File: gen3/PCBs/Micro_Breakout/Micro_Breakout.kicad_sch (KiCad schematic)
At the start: 49 parts, among them J1 BlueRobotics Depth Sensor, J10 Kill Switch, J11 StarOddi CTD Comms, J12 LED1, J13 LED2, J14 Leak Sensor, J15 Extra I2C #3, J16 Extra I2C #6, J17 Extra I2C #5, J18 Extra I2C #4, J19 GND Line, J2 Interconnect, J20 3.3V Line, J21 5V Line, J22 Extra SPI #1, J23 Extra SPI #2, J24 Extra SPI #3, J25 Secondary UART, J3 External Battery, J4 Conn_01x24, J5 External I2C, J6 Conn_01x24, J7 Extra I2C #1, J8 Extra I2C #2, J9 Lumen PWM, Q7 L78M05ABDT-TR, U1 SHT31-DIS-B, U15 AMS1117-3.3, U2 MCP9808_MSOP, U3 MS560702BA03-50, U6 Teensy4.1

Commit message: works
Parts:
- J1, J11, J15, J16, J17, J18, J25, J7, J8: footprint robosub_footprints:CONN_SD-43045-008_04_MOL -> robosub_footprints:CONN_SD-43045-005_04_MOL; symbol robosub_symbols:430450422 -> robosub_symbols:430450412; Supplier 1 https://www.digikey.com/en/products/detail/molex/0430450422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 -> https://www.digikey.com/en/products/detail/molex/0430450412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; Supplier 1 S/N WM2679-ND -> WM1790-ND
- J10, J12, J13, J9: footprint robosub_footprints:CONN_SD-43045-010_02_MOL -> robosub_footprints:CONN_SD-43045-005_02_MOL; symbol robosub_symbols:430450228 -> robosub_symbols:430450212; Supplier 1 https://www.digikey.com/en/products/detail/molex/0430450201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 -> https://www.digikey.com/en/products/detail/molex/0430450212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; Supplier 1 S/N WM9815-ND -> WM1789-ND
- J22, J23, J24: Supplier 1 (none) -> https://www.digikey.com/en/products/detail/molex/0430450612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; Supplier 1 S/N (none) -> WM1791-ND
- U6: footprint Imported_Footprints:Teensy41 -> robosub_footprints:Teensy41

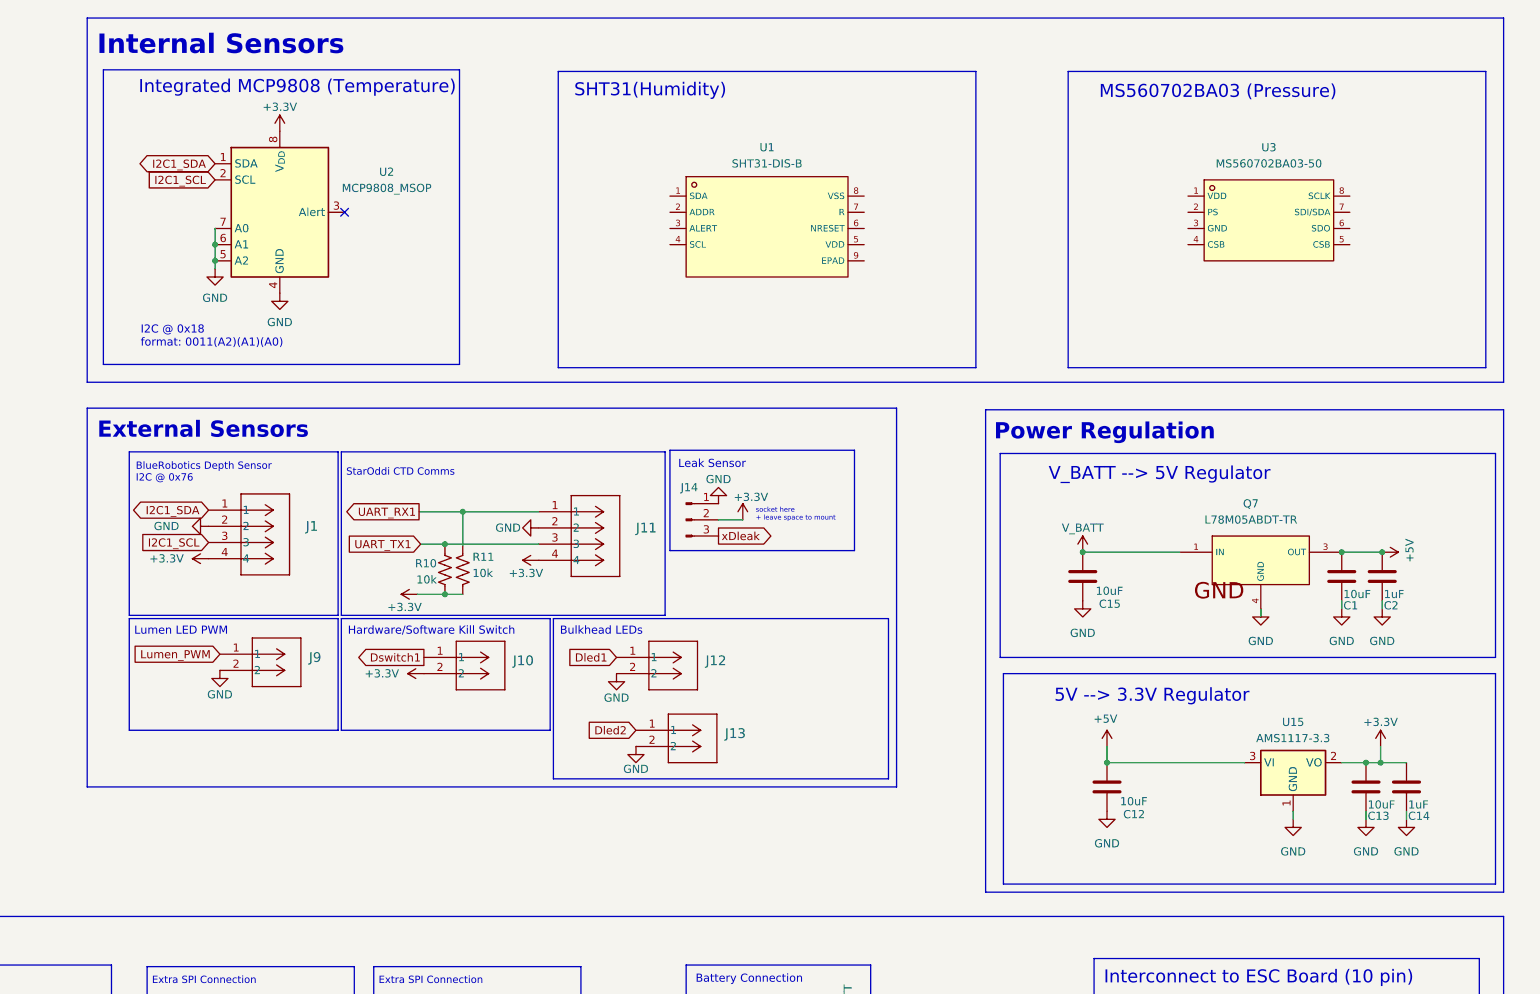
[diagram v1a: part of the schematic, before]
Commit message: jlc_to_robosub working, and all parts are updated.
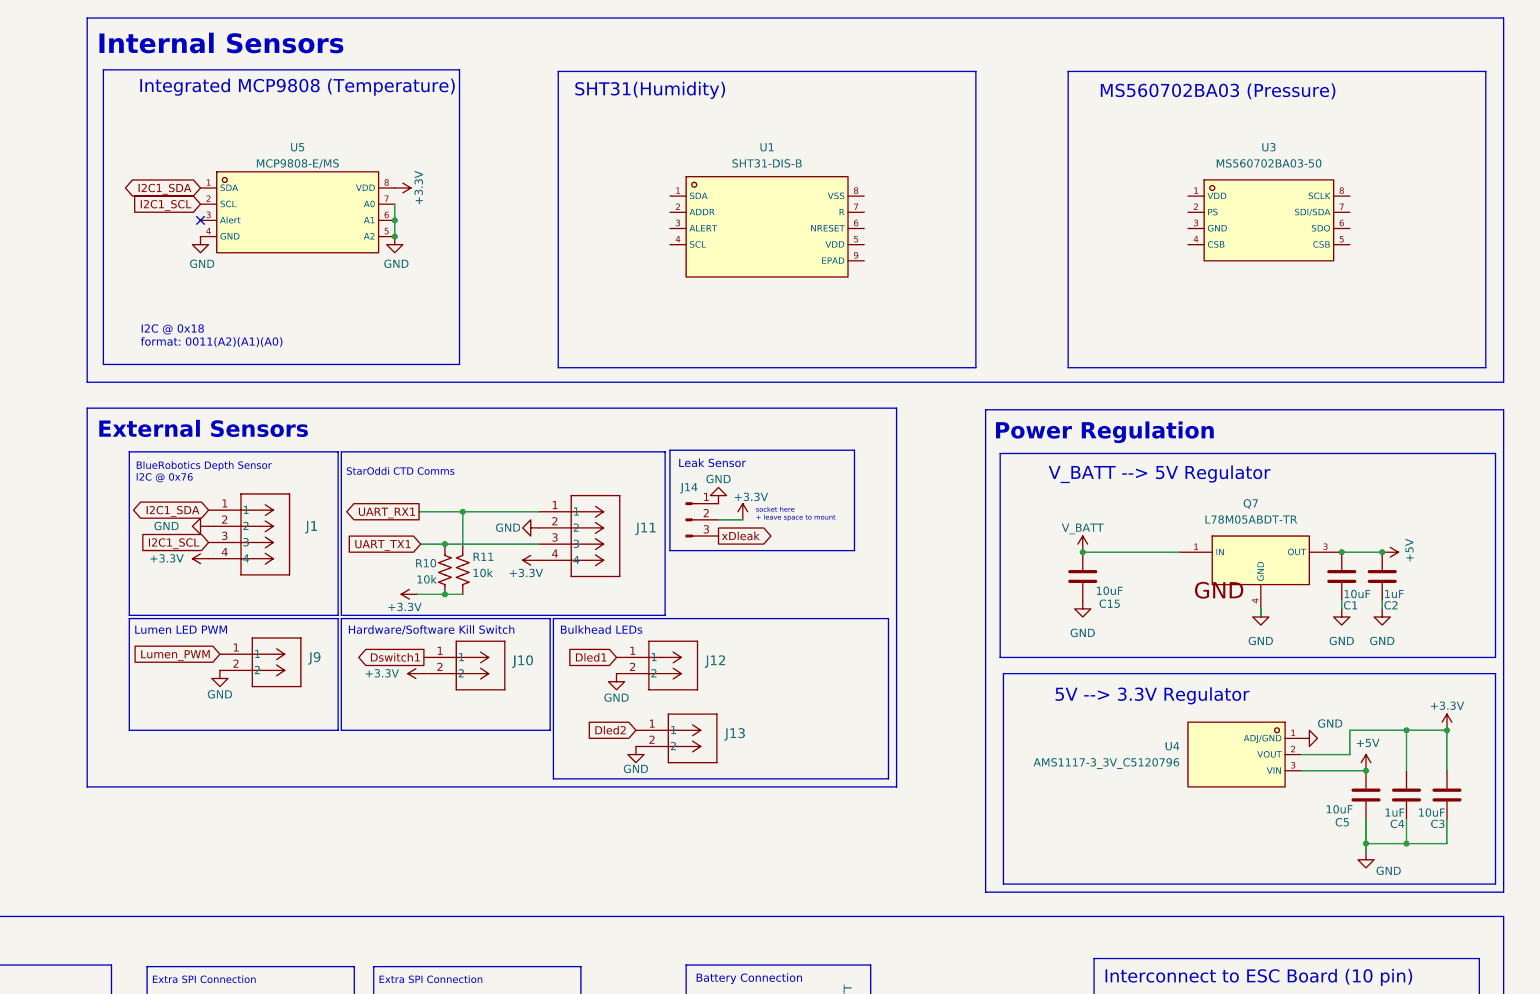
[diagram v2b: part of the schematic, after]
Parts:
- removed C12, C13: 10uF, Capacitor_SMD:C_0805_2012Metric_Pad1.18x1.45mm_HandSolder, symbol Device:C
- removed C14: 1uF, Capacitor_SMD:C_0805_2012Metric_Pad1.18x1.45mm_HandSolder, symbol Device:C
- removed U15: AMS1117-3.3, Package_TO_SOT_SMD:SOT-223-3_TabPin2, symbol Regulator_Linear:AMS1117-3.3
- removed U2: MCP9808_MSOP, Package_SO:MSOP-8_3x3mm_P0.65mm, symbol Sensor_Temperature:MCP9808_MSOP
- added C3, C5: 10uF, Capacitor_SMD:C_0805_2012Metric_Pad1.18x1.45mm_HandSolder, symbol Device:C
- added C4: 1uF, Capacitor_SMD:C_0805_2012Metric_Pad1.18x1.45mm_HandSolder, symbol Device:C
- added U4: AMS1117-3_3V_C5120796, robosub_footprints:SOT-89-3_L4.5-W2.5-P1.50-LS4.2-BR, symbol robosub_symbols:AMS1117-3_3V_C5120796
- added U5: MCP9808-E/MS, robosub_footprints:MSOP-8_L3.0-W3.0-P0.65-LS4.9-BL, symbol robosub_symbols:MCP9808-E/MS
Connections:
- net +3.3V: now also C3.1, C4.1, U4.2 (VOUT), U5.8 (VDD)
- net +5V: now also C5.1, U4.3 (VIN)
- net GND: now also C3.2, C4.2, C5.2, U4.1 (ADJ/GND), U5.4 (GND), U5.5 (A2), U5.6 (A1), U5.7 (A0)
- net I2C1_SCL: now also U5.2 (SCL)
- net I2C1_SDA: now also U5.1 (SDA)
